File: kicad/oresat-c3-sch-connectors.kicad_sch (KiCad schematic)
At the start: 15 parts, among them J1 Conn_02x26_Odd_Even, J2 Conn_02x26_Odd_Even, J7 2-1734592-0

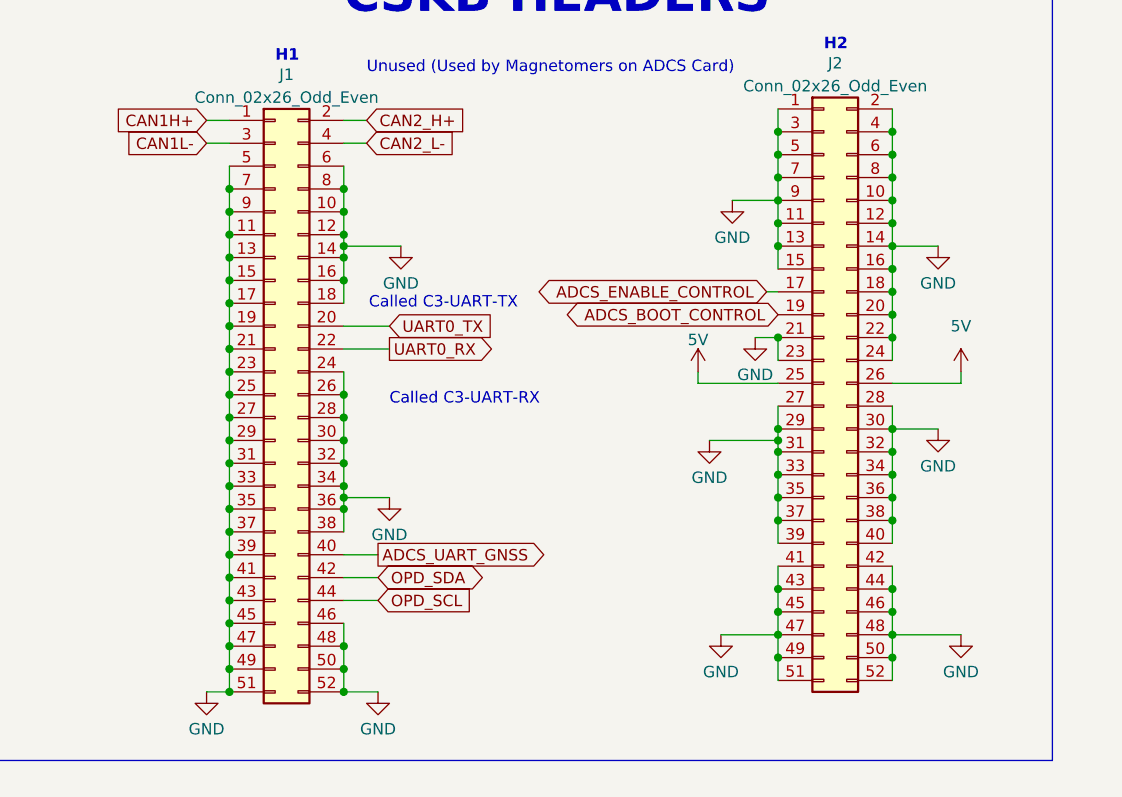
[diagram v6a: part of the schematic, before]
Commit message: Re-orientated silkscreen and added more via fencing. Also fixed BOM
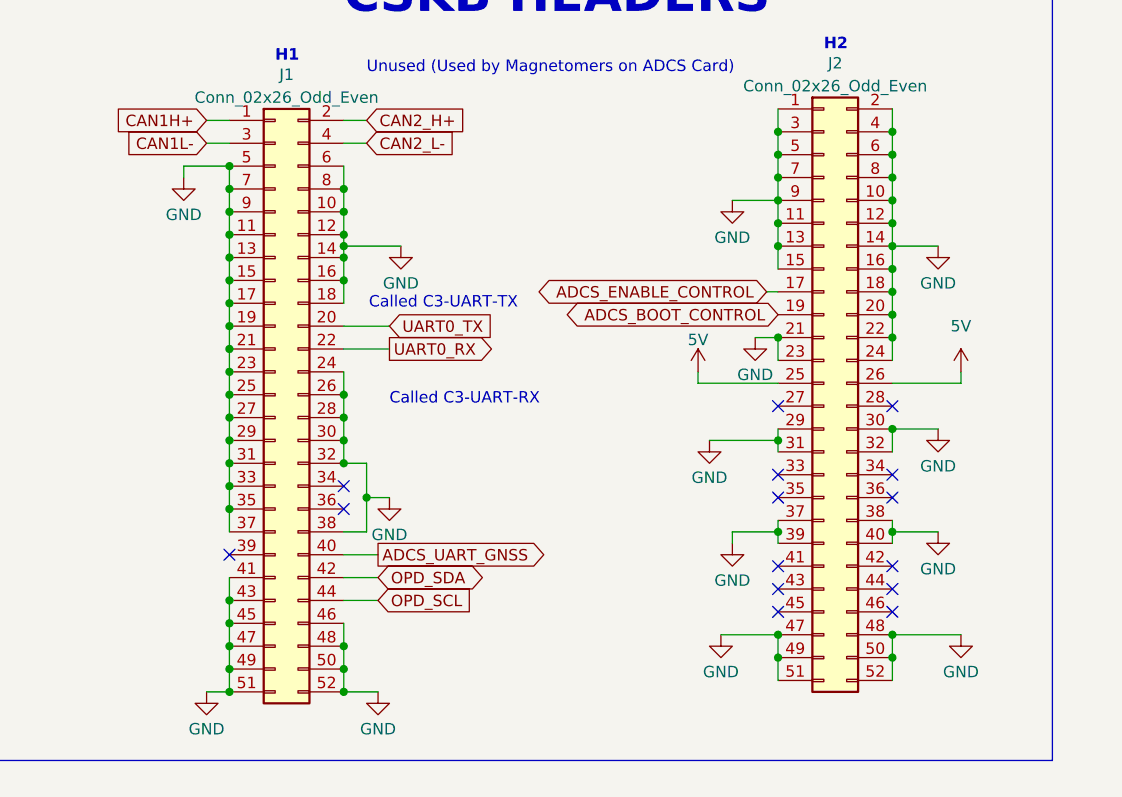
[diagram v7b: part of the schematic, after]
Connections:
- net GND: no longer J1.34 (Pin_34), J1.36 (Pin_36), J1.39 (Pin_39), J2.27 (Pin_27), J2.28 (Pin_28), J2.33 (Pin_33), J2.34 (Pin_34), J2.35 (Pin_35), J2.36 (Pin_36), J2.41 (Pin_41), J2.42 (Pin_42), J2.43 (Pin_43), J2.44 (Pin_44), J2.45 (Pin_45), J2.46 (Pin_46)
- no-connect marks 4 -> 19

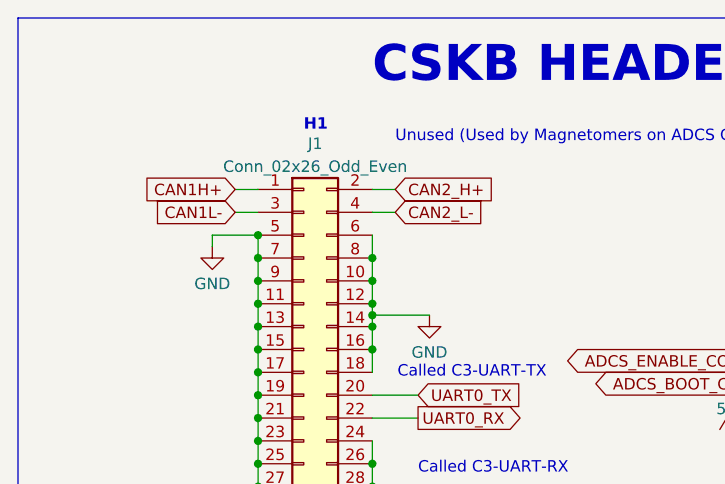
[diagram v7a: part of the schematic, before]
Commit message: Fixed skew on CAN lines
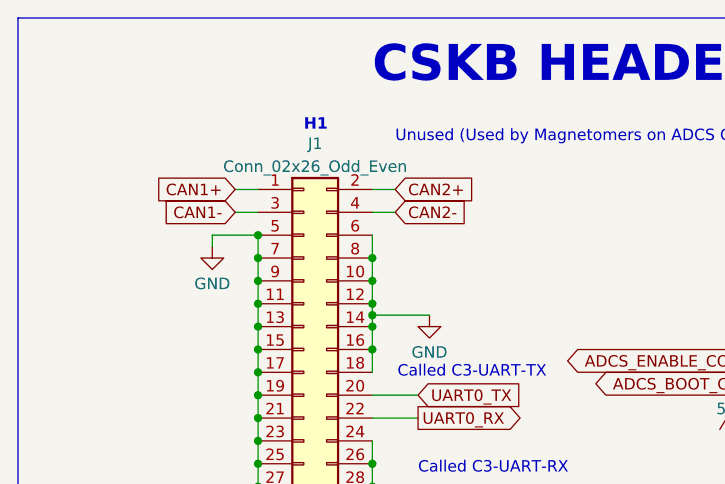
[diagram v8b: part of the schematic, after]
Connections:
- net CAN1H+ renamed CAN1+
- net CAN1L- renamed CAN1-
- net CAN2_H+ renamed CAN2+
- net CAN2_L- renamed CAN2-
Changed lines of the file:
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@@
 		)
 	)
-	(global_label "CAN2_L-"
+	(global_label "CAN2-"
 		(shape input)
 		(at 128.27 59.69 0)
@@
 		)
 		(property "Intersheetrefs" "${INTERSHEET_REFS}"
-			(at 139.7219 59.69 0)
+			(at 137.7262 59.69 0)
 			(effects
 				(font
@@
 		)
 	)
-	(global_label "CAN1H+"
+	(global_label "CAN1+"
 		(shape input)
 		(at 110.49 57.15 180)
@@
 		)
 		(property "Intersheetrefs" "${INTERSHEET_REFS}"
-			(at 99.7033 57.15 0)
+			(at 101.0338 57.15 0)
 			(effects
 				(font
@@
 		)
 	)
-	(global_label "CAN1L-"
+	(global_label "CAN1-"
 		(shape input)
 		(at 110.49 59.69 180)
@@
 		)
 		(property "Intersheetrefs" "${INTERSHEET_REFS}"
-			(at 100.0057 59.69 0)
+			(at 101.0338 59.69 0)
 			(effects
 				(font
@@
 		)
 	)
-	(global_label "CAN2_H+"
+	(global_label "CAN2+"
 		(shape input)
 		(at 128.27 57.15 0)
@@
 		)
 		(property "Intersheetrefs" "${INTERSHEET_REFS}"
-			(at 140.0243 57.15 0)
-			(effects
-				(font
+			(at 137.7262 57.15 0)
+			(effects
+				(font
